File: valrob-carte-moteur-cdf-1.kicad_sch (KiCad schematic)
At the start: 49 parts, among them J1 USB_C_Receptacle_USB2.0_14P, J2 Conn_01x02, J3 Conn_01x02, J4 Conn_01x04_Pin, J5 Conn_01x08, J6 Conn_01x02, J7 Conn_01x02, J8 Conn_01x08, SW1 SW_Push, SW2 SW_Push, U1 AP2112K-3.3, U2 USBLC6-2SC6, U3 ESP32-S3-WROOM-1

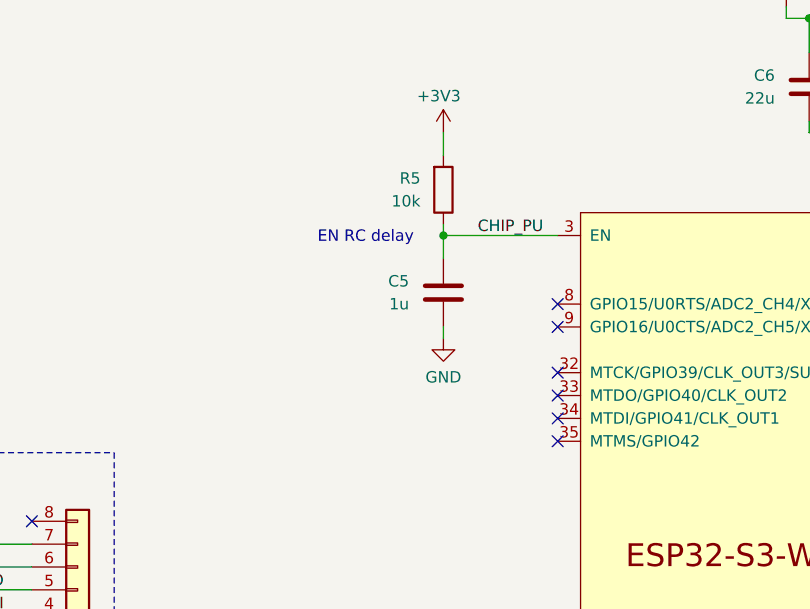
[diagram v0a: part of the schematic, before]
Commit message: add spare gpios
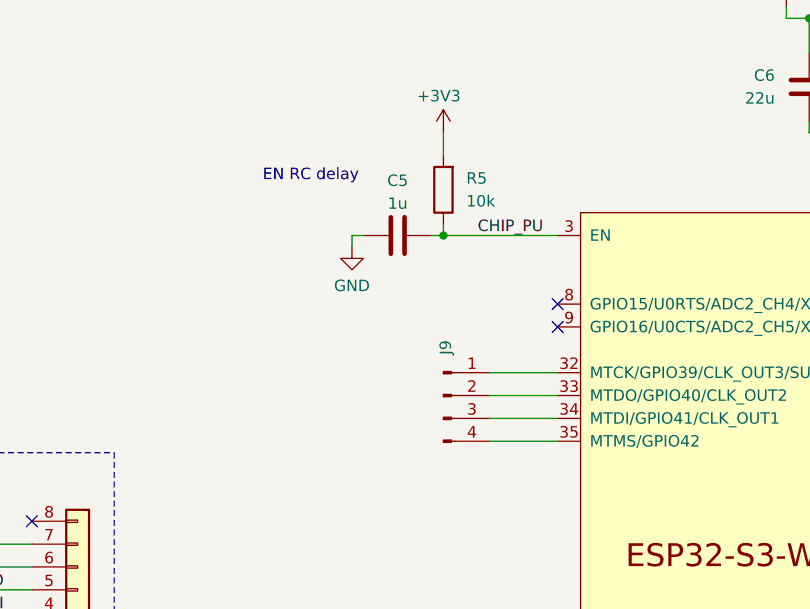
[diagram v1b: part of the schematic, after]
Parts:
- added J9: Conn_01x04_Pin, Connector_PinHeader_2.54mm:PinHeader_1x04_P2.54mm_Vertical, symbol Connector:Conn_01x04_Pin
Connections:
- net CHIP_PU: now also C5.2; no longer C5.1
- net GND: now also C5.1; no longer C5.2
- net at U3.32 (MTCK/GPIO39/CLK_OUT3/SUBSPICS1): now also J9.1 (Pin_1)
- net at U3.33 (MTDO/GPIO40/CLK_OUT2): now also J9.2 (Pin_2)
- net at U3.34 (MTDI/GPIO41/CLK_OUT1): now also J9.3 (Pin_3)
- net at U3.35 (MTMS/GPIO42): now also J9.4 (Pin_4)
- no-connect marks 15 -> 11
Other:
- moved on the sheet: C5, R5
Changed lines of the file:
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@@
 	(text "EN RC delay"
 		(exclude_from_sim no)
-		(at 122.174 53.594 0)
+		(at 116.078 46.736 0)
 		(effects
 			(font
@@
 	)
 	(no_connect
-		(at 143.51 73.66)
-	)
-	(no_connect
 		(at 234.95 78.74)
 	)
@@
 		(at 45.72 85.09)
 	)
-	(no_connect
-		(at 143.51 68.58)
-	)
-	(no_connect
-		(at 143.51 76.2)
-	)
-	(no_connect
-		(at 143.51 71.12)
-	)
 	(wire
 		(pts
@@
 	(wire
 		(pts
-			(xy 130.81 53.34) (xy 130.81 55.88)
-		)
-		(stroke
-			(width 0)
-			(type default)
-		)
-	)
-	(wire
-		(pts
 			(xy 114.3 181.61) (xy 114.3 180.34)
 		)
@@
 	(wire
 		(pts
+			(xy 143.51 73.66) (xy 135.89 73.66)
+		)
+		(stroke
+			(width 0)
+			(type default)
+		)
+	)
+	(wire
+		(pts
 			(xy 60.96 110.49) (xy 64.77 110.49)
 		)
@@
 	(wire
 		(pts
+			(xy 120.65 54.61) (xy 120.65 53.34)
+		)
+		(stroke
+			(width 0)
+			(type default)
+		)
+	)
+	(wire
+		(pts
 			(xy 238.76 116.84) (xy 238.76 109.22)
 		)
@@
 	(wire
 		(pts
+			(xy 143.51 71.12) (xy 135.89 71.12)
+		)
+		(stroke
+			(width 0)
+			(type default)
+		)
+	)
+	(wire
+		(pts
 			(xy 40.64 111.76) (xy 40.64 110.49)
 		)
@@
 	(wire
 		(pts
+			(xy 120.65 53.34) (xy 121.92 53.34)
+		)
+		(stroke
+			(width 0)
+			(type default)
+		)
+	)
+	(wire
+		(pts
 			(xy 130.81 53.34) (xy 143.51 53.34)
 		)
@@
 	(wire
 		(pts
-			(xy 130.81 63.5) (xy 130.81 64.77)
-		)
-		(stroke
-			(width 0)
-			(type default)
-		)
-	)
-	(wire
-		(pts
 			(xy 132.08 185.42) (xy 134.62 185.42)
 		)
@@
 	(wire
 		(pts
+			(xy 143.51 68.58) (xy 135.89 68.58)
+		)
+		(stroke
+			(width 0)
+			(type default)
+		)
+	)
+	(wire
+		(pts
 			(xy 44.45 128.27) (xy 44.45 129.54)
 		)
@@
 	(wire
 		(pts
+			(xy 129.54 53.34) (xy 130.81 53.34)
+		)
+		(stroke
+			(width 0)
+			(type default)
+		)
+	)
+	(wire
+		(pts
 			(xy 234.95 81.28) (xy 242.57 81.28)
 		)
@@
 	(wire
 		(pts
+			(xy 143.51 76.2) (xy 135.89 76.2)
+		)
+		(stroke
+			(width 0)
+			(type default)
+		)
+	)
+	(wire
+		(pts
 			(xy 45.72 170.18) (xy 53.34 170.18)
 		)
@@
 	(symbol
 		(lib_id "Device:C")
-		(at 130.81 59.69 0)
-		(mirror y)
+		(at 125.73 53.34 90)
+		(mirror x)
 		(unit 1)
 		(exclude_from_sim no)
@@
 		(dnp no)
 		(property "Reference" "C5"
-			(at 127 58.4199 0)
+			(at 125.73 47.244 90)
 			(effects
 				(font
 					(size 1.27 1.27)
 				)
-				(justify left)
 			)
 		)
 		(property "Value" "1u"
-			(at 127 60.9599 0)
+			(at 125.73 49.784 90)
 			(effects
 				(font
 					(size 1.27 1.27)
 				)
-				(justify left)
 			)
 		)
 		(property "Footprint" "Capacitor_SMD:C_0603_1608Metric"
-			(at 129.8448 63.5 0)
+			(at 129.54 54.3052 0)
 			(effects
 				(font
@@
 		)
 		(property "Datasheet" "~"
-			(at 130.81 59.69 0)
+			(at 125.73 53.34 0)
 			(effects
 				(font
@@
 		)
 		(property "Description" "Unpolarized capacitor"
-			(at 130.81 59.69 0)
+			(at 125.73 53.34 0)
 			(effects
 				(font
@@
 		)
 		(property "Manufacturer" "Samsung Electro-Mechanics "
-			(at 130.81 59.69 0)
+			(at 125.73 53.34 0)
 			(effects
 				(font
@@
 		)
 		(property "Manufacturer Part Number" "CL10A105KB8NNNC"
-			(at 130.81 59.69 0)
+			(at 125.73 53.34 0)
 			(effects
 				(font
@@
 		)
 		(property "Basic" "Y"
-			(at 130.81 59.69 0)
+			(at 125.73 53.34 0)
 			(effects
 				(font
@@
 		)
 		(property "JLCPCB Part #" "C15849"
-			(at 130.81 59.69 0)
+			(at 125.73 53.34 0)
 			(effects
 				(font
@@
 	(symbol
 		(lib_id "Device:R")
-		(at 130.81 48.26 0)
-		(mirror x)
+		(at 130.81 48.26 180)
 		(unit 1)
 		(exclude_from_sim no)
@@
 		(dnp no)
 		(property "Reference" "R5"
-			(at 128.27 46.9899 0)
+			(at 133.35 46.9899 0)
 			(effects
 				(font
@@
 		)
 		(property "Value" "10k"
-			(at 128.27 49.5299 0)
+			(at 133.35 49.5299 0)
 			(effects
 				(font
@@
 		)
 		(property "Footprint" "Resistor_SMD:R_0603_1608Metric"
-			(at 129.032 48.26 90)
+			(at 132.588 48.26 90)
 			(effects
 				(font
@@
 	(symbol
 		(lib_id "power:GND")
-		(at 130.81 64.77 0)
+		(at 120.65 54.61 0)
 		(unit 1)
 		(exclude_from_sim no)
@@
 		(dnp no)
 		(property "Reference" "#PWR018"
-			(at 130.81 71.12 0)
+			(at 120.65 60.96 0)
 			(effects
 				(font
@@
 		)
 		(property "Value" "GND"
-			(at 130.81 69.088 0)
+			(at 120.65 58.928 0)
 			(effects
 				(font
@@
 		)
 		(property "Footprint" ""
-			(at 130.81 64.77 0)
+			(at 120.65 54.61 0)
 			(effects
 				(font
@@
 		)
 		(property "Datasheet" ""
-			(at 130.81 64.77 0)
+			(at 120.65 54.61 0)
 			(effects
 				(font
@@
 		)
 		(property "Description" "Power symbol creates a global label with name \"GND\" , ground"
-			(at 130.81 64.77 0)
+			(at 120.65 54.61 0)
 			(effects
 				(font
@@
 					(unit 1)
 				)
+			)
+		)
+	)
+	(symbol
+		(lib_id "Connector:Conn_01x04_Pin")
+		(at 130.81 71.12 0)
+		(unit 1)
+		(exclude_from_sim no)
+		(in_bom no)
+		(on_board yes)
+		(dnp no)
+		(property "Reference" "J9"
+			(at 131.064 65.786 90)
+			(effects
+				(font
+					(size 1.27 1.27)
+				)
+			)
+		)
+		(property "Value" "Conn_01x04_Pin"
+			(at 128.27 72.39 90)
+			(effects
+				(font
+					(size 1.27 1.27)
+				)
+				(hide yes)
+			)
+		)
+		(property "Footprint" "Connector_PinHeader_2.54mm:PinHeader_1x04_P2.54mm_Vertical"
+			(at 130.81 71.12 0)
+			(effects
+				(font
+					(size 1.27 1.27)
+				)
+				(hide yes)
+			)
+		)
+		(property "Datasheet" "~"
+			(at 130.81 71.12 0)
+			(effects
+				(font
+					(size 1.27 1.27)
+				)
+				(hide yes)
+			)
+		)
+		(property "Description" "Generic connector, single row, 01x04, script generated"
+			(at 130.81 71.12 0)
+			(effects
+				(font
+					(size 1.27 1.27)
+				)
+				(hide yes)
+			)
+		)
+		(pin "4"
+		)
+		(pin "3"
+		)
+		(pin "2"
+		)
+		(pin "1"
+		)
+		(instances
+			(project "valrob-carte-moteur-cdf-1"
+				(path "/b89f538c-def5-4450-bb35-40e96c574400"
+					(reference "J9")
+					(unit 1)
+				)
